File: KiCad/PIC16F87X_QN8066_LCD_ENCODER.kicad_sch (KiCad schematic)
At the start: 17 parts, among them J1 Conn_01x05_Socket, SW1 RotaryEncoder_Switch, U1 PIC16F876-XXISO, U2 LCD-016N002L, U3 DS1302+, Y1 8MHz, Y2 32.768kHz

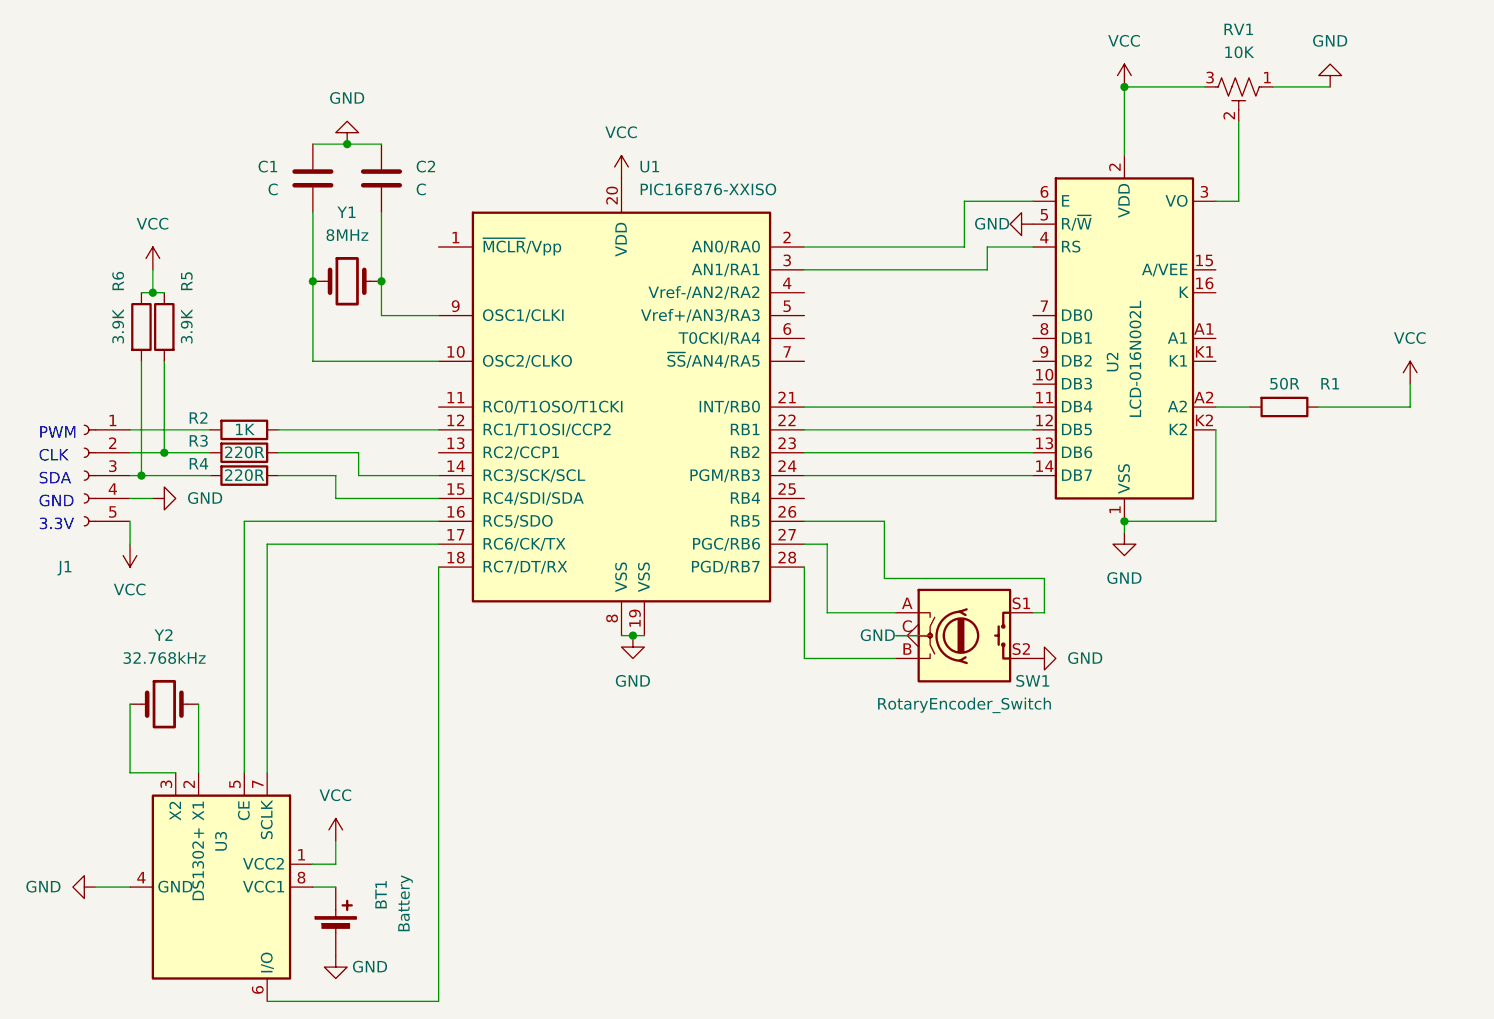
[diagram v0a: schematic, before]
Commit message: Doc
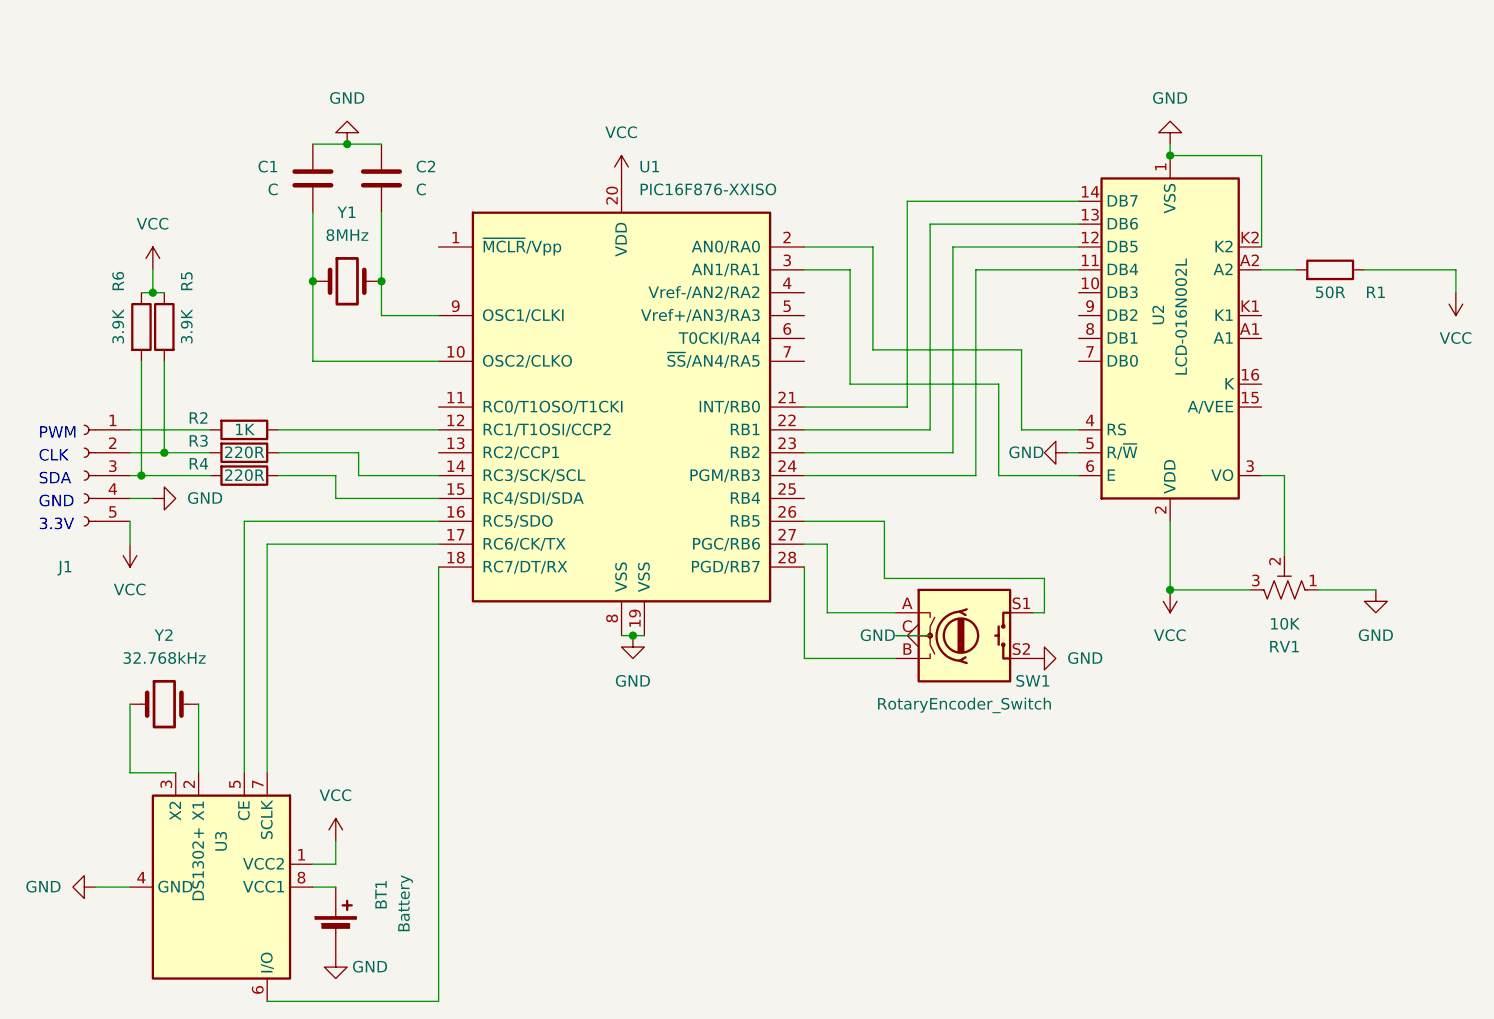
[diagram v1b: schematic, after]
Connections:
- net at U2.11 (DB4): now also U1.24 (PGM/RB3); no longer U1.21 (INT/RB0)
- net at U2.12 (DB5): now also U1.23 (RB2); no longer U1.22 (RB1)
- net at U2.13 (DB6): now also U1.22 (RB1); no longer U1.23 (RB2)
- net at U2.14 (DB7): now also U1.21 (INT/RB0); no longer U1.24 (PGM/RB3)
- net at U2.4 (RS): now also U1.2 (AN0/RA0); no longer U1.3 (AN1/RA1)
- net at U2.6 (E): now also U1.3 (AN1/RA1); no longer U1.2 (AN0/RA0)
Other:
- moved on the sheet: R1, RV1, U2
